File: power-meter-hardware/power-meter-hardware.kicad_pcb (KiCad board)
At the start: 2 copper layers, 80 x 150 mm, 27 parts, among them J1 Jack-DC, J2 LOAD_DISCONNECT, K1 FINDER-36.11, Q1 BC548, SW1 SW_SPST, U1 LM2596, U2 AMS1117-3.3, U3 NodeMCU, U4 SSD1306_OLED_SCREEN_0.91, U5 ACS712, U6 LM7805_TO220, U7 LM2596

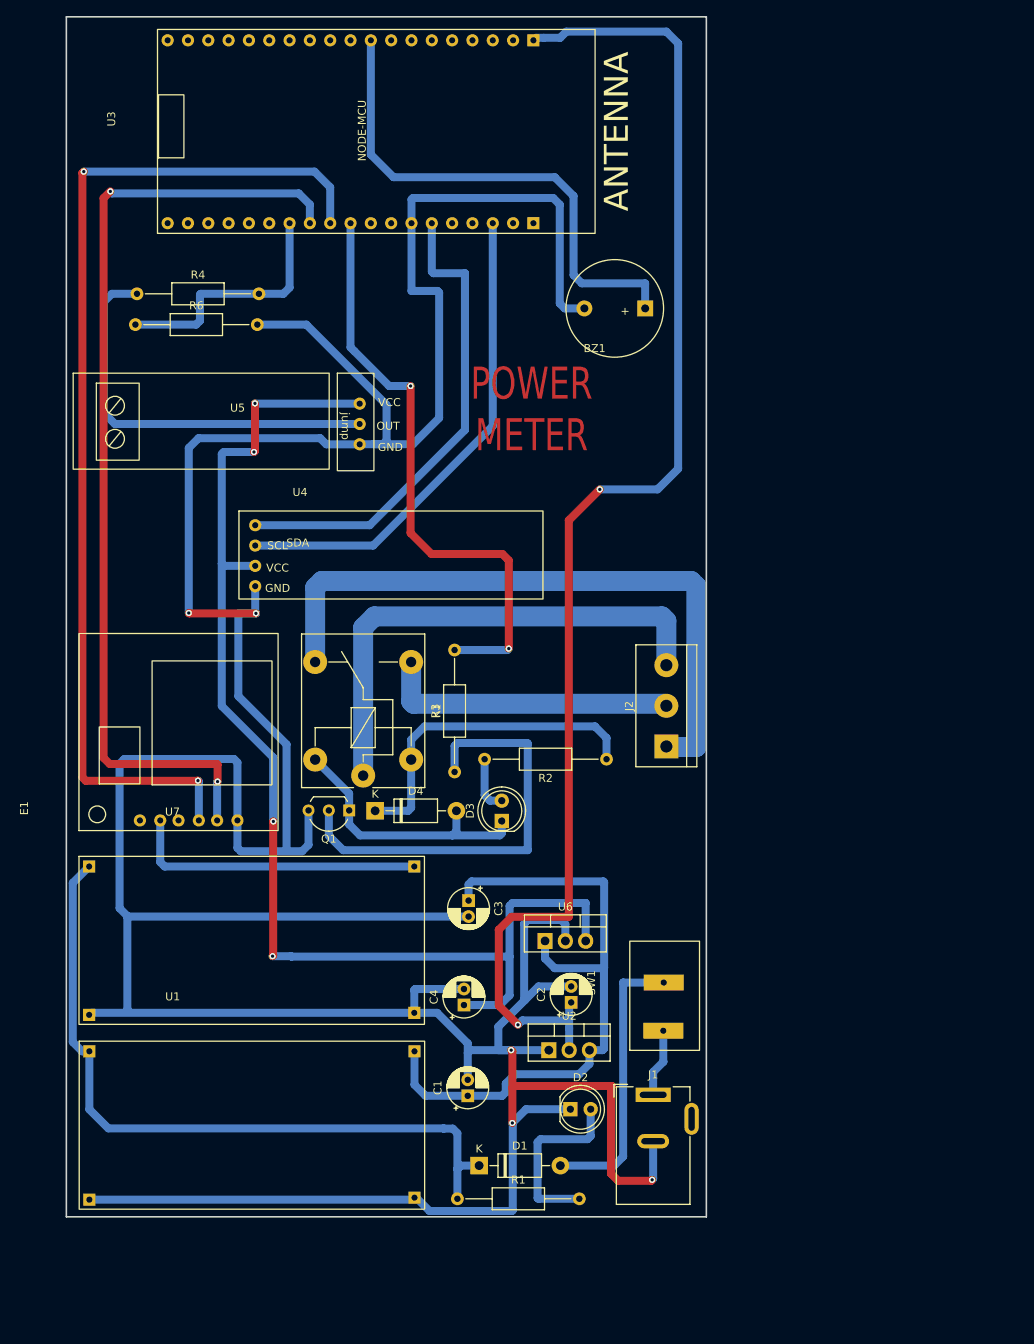
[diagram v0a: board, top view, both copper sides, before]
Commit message: added flowcharts
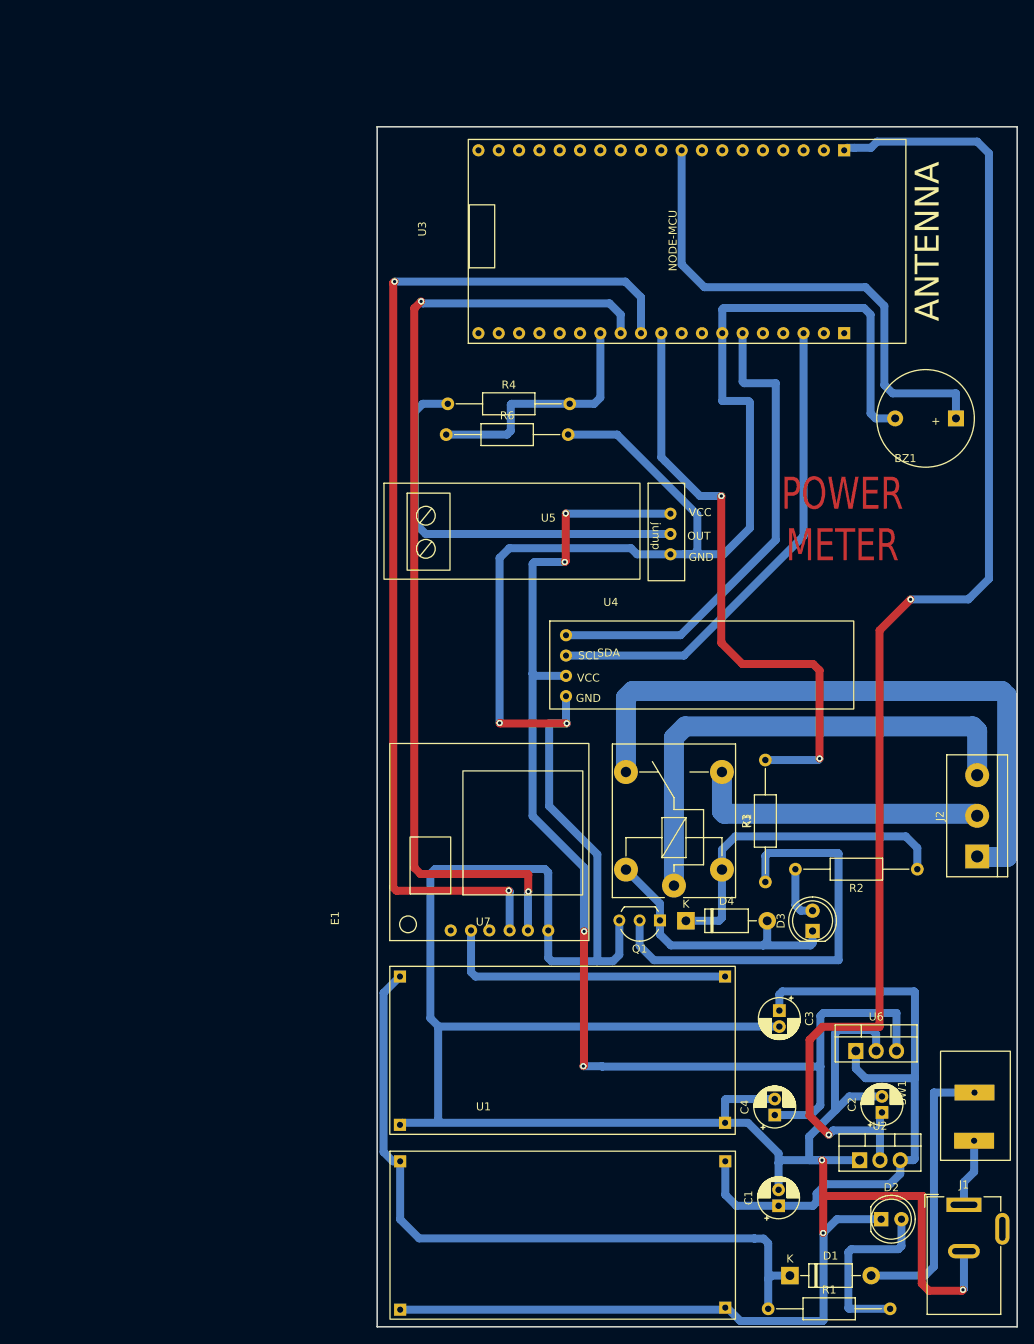
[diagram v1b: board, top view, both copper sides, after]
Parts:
- moved BZ1 41.2 mm to (127.5, 66.1)
- moved C1 41.2 mm to (105.3, 164.5)
- moved C2 41.2 mm to (118.2, 152.8)
- moved D3 41.2 mm to (109.5, 130.2)
- moved R1 41.2 mm to (104.0, 177.4)
- moved R2 41.2 mm to (122.6, 122.4)
- moved U6 41.2 mm to (114.9, 145.1)
- moved K1 41.2 mm to (92.2, 124.5)
- moved Q1 41.2 mm to (90.5, 128.8)
- moved R4 41.2 mm to (63.9, 64.2)
- moved U5 41.2 mm to (55.9, 74.2)
- moved U7 41.2 mm to (56.7, 134.6)
- moved C3 41.2 mm to (105.4, 140.1)
- moved C4 41.2 mm to (104.8, 153.2)
- moved D1 41.2 mm to (106.7, 173.2)
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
